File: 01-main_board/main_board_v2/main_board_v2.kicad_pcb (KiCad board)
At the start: 4 copper layers, 93.5 x 62.8 mm, 158 parts, among them IC1 MAX6105EUR+T, IC10 ESP32-S3, IC11 LT3973EMSE-5#PBF, IC2 LP5907MFX-2.5_NOPB, IC3 TS3USB30EDGSR, IC4 SPX3819S-L_TR, IC5 INA827AIDGK, IC6 AD7175-8BCPZ-RL7, IC7 INA827AIDGK, IC8 AD8591ARTZ-REEL7, IC9 LSF0108PWR, J2 DF12NB-20DS-0.5V_51_, J4 DB44 (Analog | Digital), T1 749013011, U1 Teensy4.1, U2 AD5689RARUZ-RL7, U3 MCP2562FD-E/SN, U4 TPS2115APWR, Y1 ECS-400-10-37B2-CKY-TR, Y2 ECS-.327-12.5-34B-TR

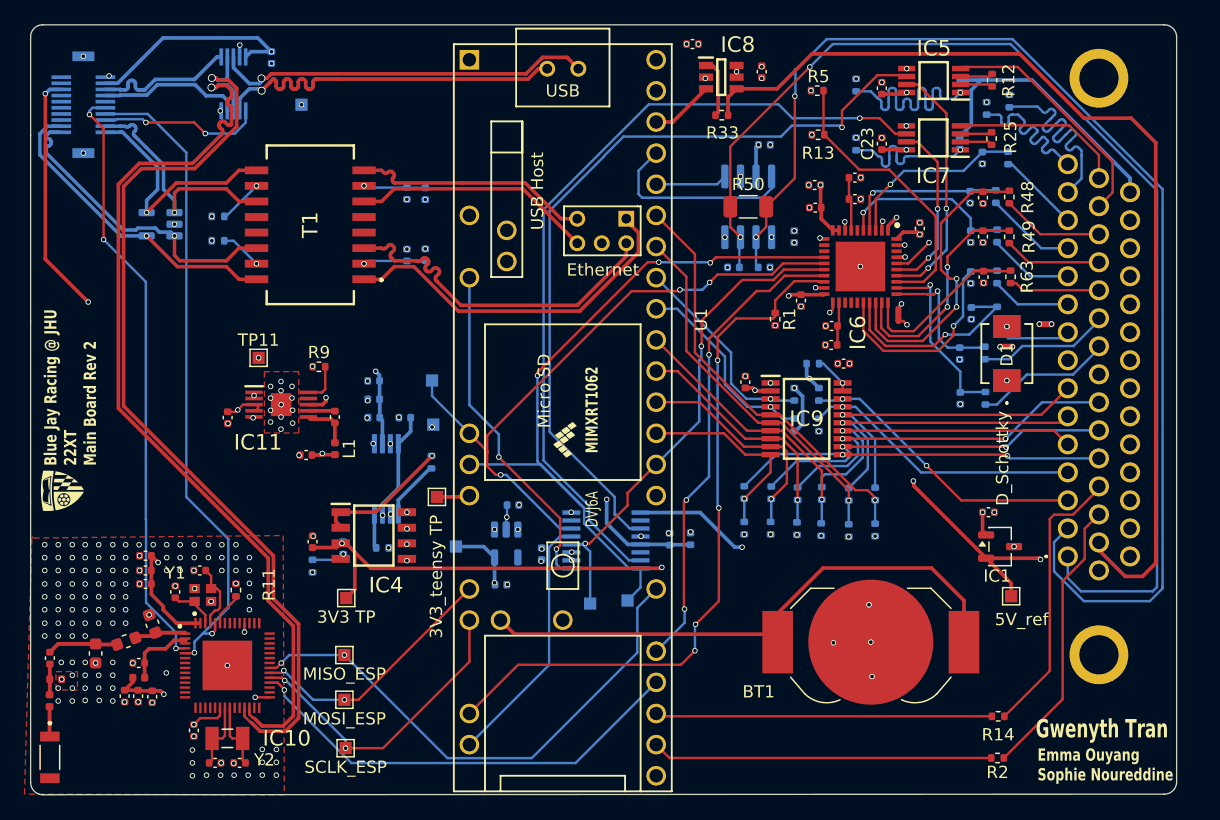
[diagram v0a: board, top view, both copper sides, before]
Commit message: dimensions finalized
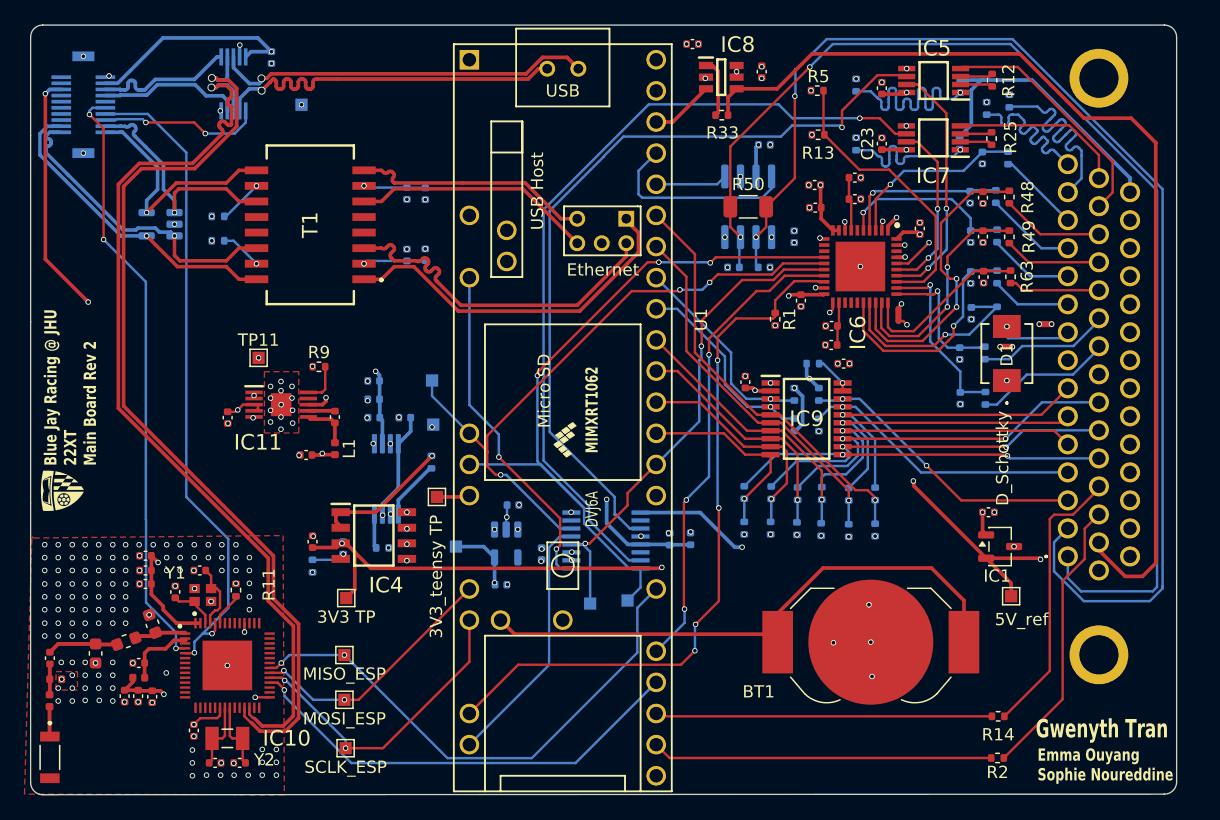
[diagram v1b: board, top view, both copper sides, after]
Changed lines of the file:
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@@
 	)
 	(gr_line
-		(start 137.9 82.449999)
-		(end 137.899949 21.67995)
-		(stroke
-			(width 0.05)
-			(type default)
-		)
-		(layer "Edge.Cuts")
-	)
-	(gr_arc
-		(start 136.9 20.67995)
-		(mid 137.607089 20.972846)
-		(end 137.9 21.67995)
+		(start 137.9 82.45)
+		(end 137.899949 21.7)
+		(stroke
+			(width 0.05)
+			(type default)
+		)
+		(layer "Edge.Cuts")
+	)
+	(gr_arc
+		(start 136.9 20.7)
+		(mid 137.607124 20.99289)
+		(end 137.9 21.7)
 		(stroke
 			(width 0.05)
@@
 	)
 	(gr_line
-		(start 44.4 21.657103)
+		(start 44.4 21.677153)
 		(end 44.4 29.7)
 		(stroke
@@
 	)
 	(gr_line
-		(start 136.9 20.67995)
-		(end 45.377104 20.67995)
+		(start 136.9 20.7)
+		(end 45.377104 20.7)
 		(stroke
 			(width 0.05)
@@
 	)
 	(gr_arc
-		(start 44.4 21.657103)
-		(mid 44.68617 20.966154)
-		(end 45.377104 20.67995)
+		(start 44.4 21.677153)
+		(mid 44.686186 20.986236)
+		(end 45.377104 20.7)
 		(stroke
 			(width 0.05)
@@
 		(layer "Dwgs.User")
 		(pts
-			(xy 136.9 20.67995) (xy 136.9 83.45)
-		)
-		(height 6.3)
+			(xy 136.9 20.7) (xy 136.9 83.45)
+		)
+		(height 6.4)
 		(orientation 1)
 		(format
@@
 			(keep_text_aligned yes)
 		)
-		(gr_text "62.77"
-			(at 142.05 52.064975 90)
+		(gr_text "62.75"
+			(at 142.15 52.075 90)
 			(layer "Dwgs.User")
 			(effects
